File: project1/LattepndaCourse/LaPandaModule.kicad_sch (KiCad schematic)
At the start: 1 part

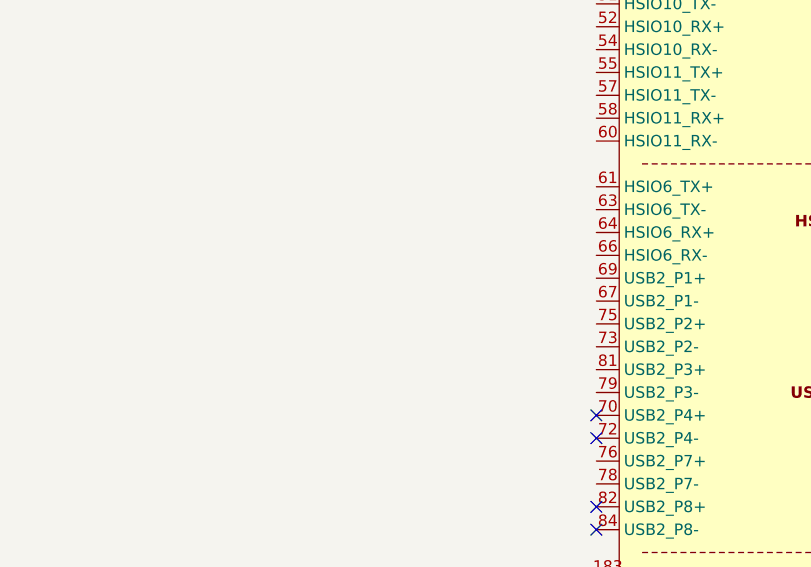
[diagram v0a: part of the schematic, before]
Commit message: test2
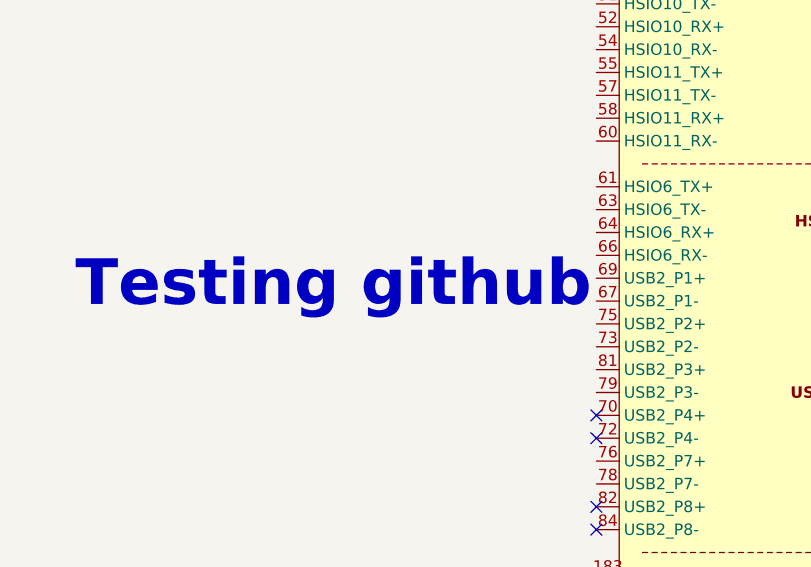
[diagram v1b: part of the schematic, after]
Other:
- note added: "Testing github"
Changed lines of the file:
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@@
 (kicad_sch
-	(version 20250114)
+	(version 20260306)
 	(generator "eeschema")
-	(generator_version "9.0")
+	(generator_version "10.0")
 	(paper "A2")
 	(title_block
@@
 		(rev "1")
 	)
+	(text "Testing github"
+		(exclude_from_sim no)
+		(at 226.06 181.102 0)
+		(effects
+			(font
+				(size 5.08 5.08)
+				(thickness 1.016)
+				(bold yes)
+				(color 255 51 215 1)
+			)
+		)
+	)
 	(no_connect
 		(at 255.27 195.58)
@@
 		(at 295.91 195.58 0)
 		(unit 1)
+		(body_style 1)
 		(exclude_from_sim no)
 		(in_bom yes)
 		(on_board yes)
+		(in_pos_files yes)
 		(dnp no)
 		(fields_autoplaced yes)
 		(property "Reference" "A1"
 			(at 300.5933 58.42 0)
+			(show_name no)
+			(do_not_autoplace no)
 			(effects
 				(font
@@
 		(property "Value" "LattePanda_Mu"
 			(at 300.5933 60.96 0)
+			(show_name no)
+			(do_not_autoplace no)
 			(effects
 				(font
@@
 		(property "Footprint" "Module_LattePanda:LattePanda_Module_H8.0mm_Horizontal"
 			(at 295.91 185.42 0)
+			(hide yes)
+			(show_name no)
+			(do_not_autoplace no)
 			(effects
 				(font
 					(size 1.27 1.27)
 				)
-				(hide yes)
 			)
 		)
 		(property "Datasheet" ""
 			(at 295.91 185.42 0)
+			(hide yes)
+			(show_name no)
+			(do_not_autoplace no)
 			(effects
 				(font
 					(size 1.27 1.27)
 				)
-				(hide yes)
 			)
 		)
 		(property "Description" "A micro computing module with x86 processer, RAM and eMMC."
 			(at 295.91 195.58 0)
+			(hide yes)
+			(show_name no)
+			(do_not_autoplace no)
 			(effects
 				(font
 					(size 1.27 1.27)
 				)
-				(hide yes)
 			)
 		)
@@
 		)
 		(instances
-			(project ""
+			(project "LattepndaCourse"
 				(path "/4e04f3a7-ba43-4db9-8bbc-1a27efcf5abf/e658b8ed-bbad-487b-848e-8e04e48b43c0"
 					(reference "A1")

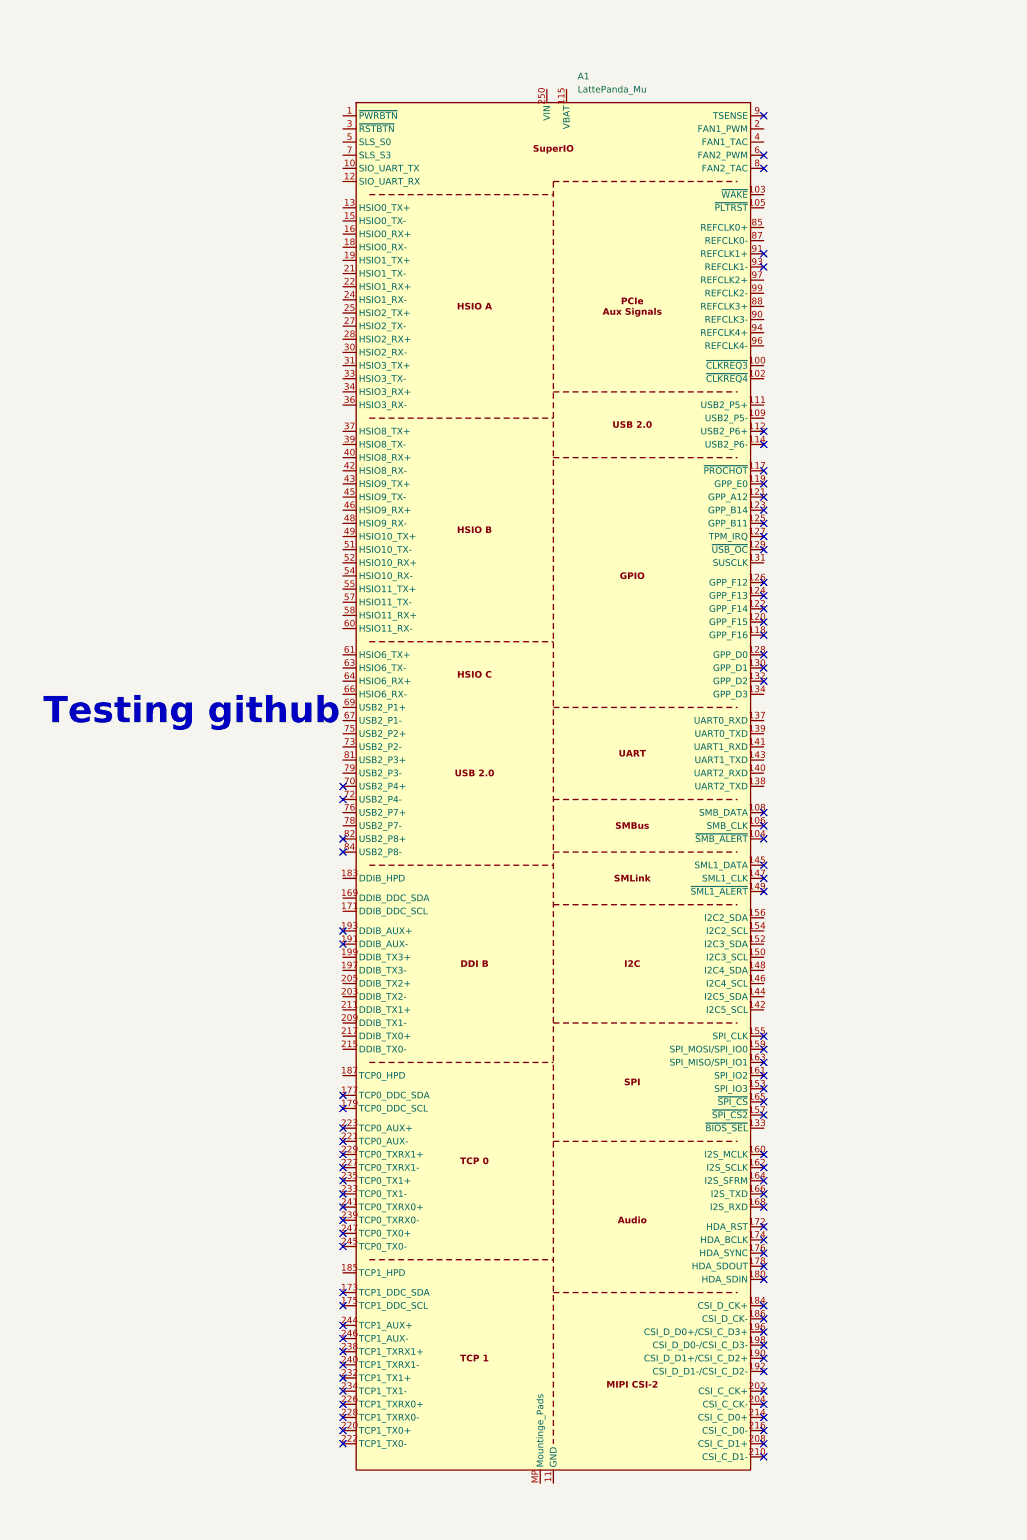
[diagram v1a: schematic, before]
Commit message: 9/30/36 10pm
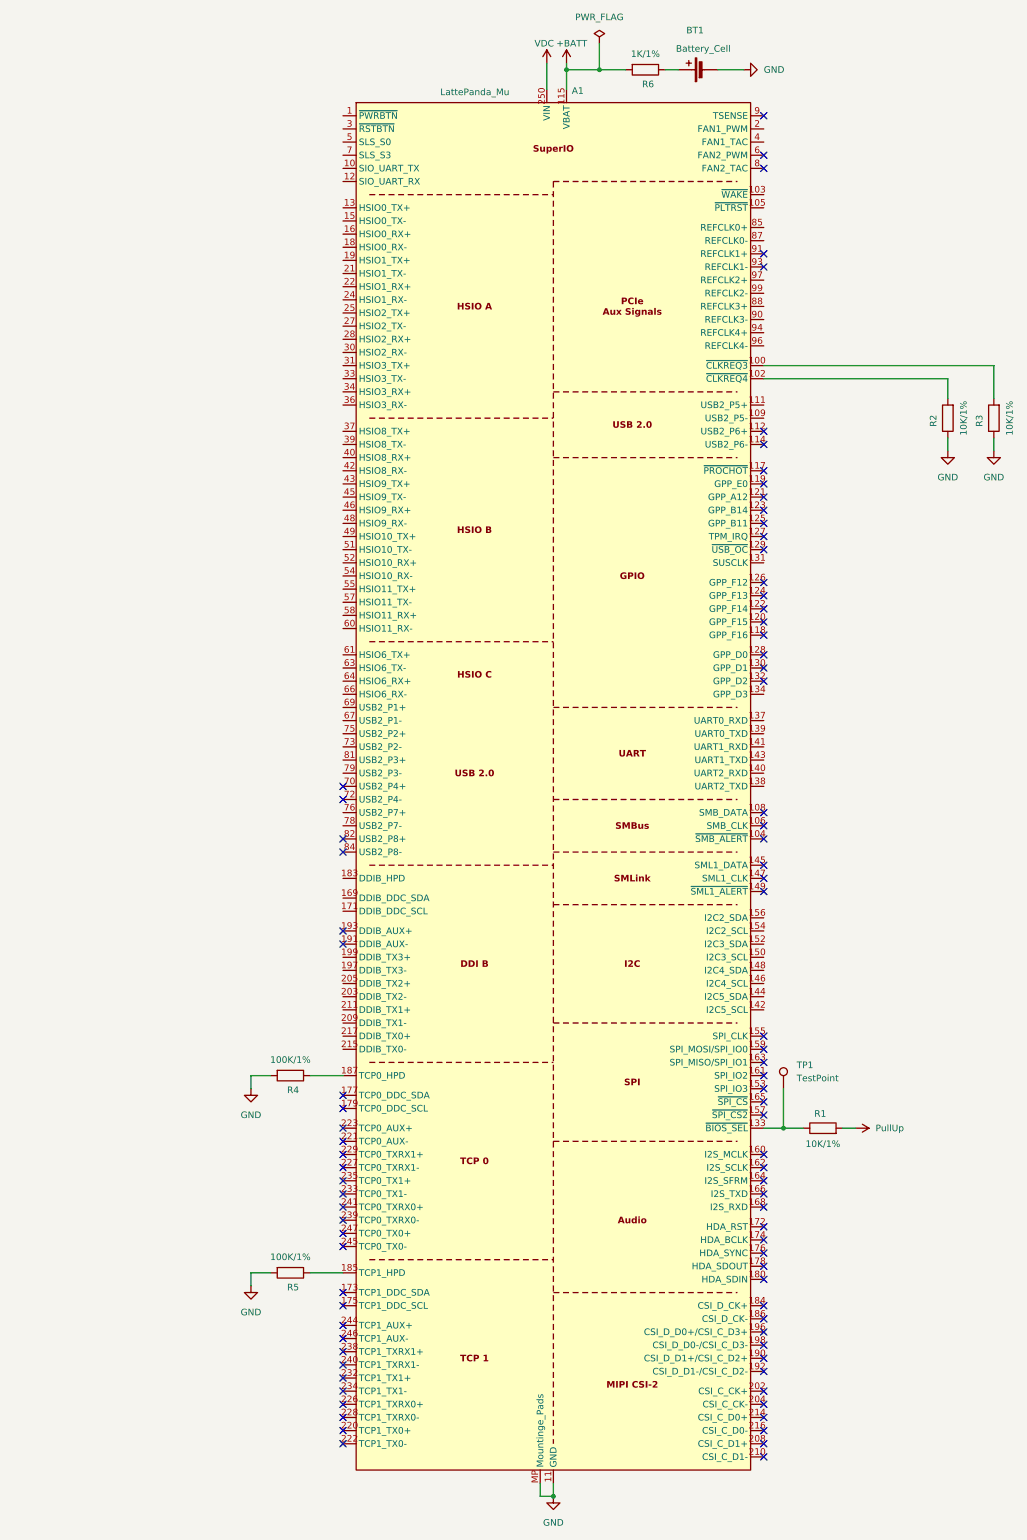
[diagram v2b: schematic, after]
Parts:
- added BT1: Battery_Cell, symbol Device:Battery_Cell
- added R1, R2, R3: 10K/1%, symbol Device:R
- added R4, R5: 100K/1%, symbol Device:R
- added R6: 1K/1%, symbol Device:R
- added TP1: TestPoint, symbol Connector:TestPoint
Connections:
- net at A1.100 (~{CLKREQ3}): now also R3.2
- net GND: now reaches A1.101 (GND), A1.107 (GND), A1.11 (GND), A1.110 (GND), A1.113 (GND), A1.116 (GND), A1.135 (GND), A1.136 (GND), A1.14 (GND), A1.151 (GND), A1.158 (GND), A1.167 (GND), A1.17 (GND), A1.170 (GND), A1.181 (GND), A1.182 (GND), A1.188 (GND), A1.189 (GND), A1.194 (GND), A1.195 (GND), A1.20 (GND), A1.200 (GND), A1.201 (GND), A1.206 (GND), A1.207 (GND), A1.212 (GND), A1.213 (GND), A1.218 (GND), A1.219 (GND), A1.224 (GND), A1.225 (GND), A1.23 (GND), A1.230 (GND), A1.231 (GND), A1.236 (GND), A1.237 (GND), A1.242 (GND), A1.243 (GND), A1.248 (GND), A1.249 (GND), A1.26 (GND), A1.29 (GND), A1.32 (GND), A1.35 (GND), A1.38 (GND), A1.41 (GND), A1.44 (GND), A1.47 (GND), A1.50 (GND), A1.53 (GND), A1.56 (GND), A1.59 (GND), A1.62 (GND), A1.65 (GND), A1.68 (GND), A1.71 (GND), A1.74 (GND), A1.77 (GND), A1.80 (GND), A1.83 (GND), A1.86 (GND), A1.89 (GND), A1.92 (GND), A1.95 (GND), A1.98 (GND)
- net GND: now also A1.MP (Mountinge_Pads), BT1.2 (-), R2.1, R3.1, R4.2, R5.2
- net at A1.102 (~{CLKREQ4}): now also R2.2
- net +BATT: now reaches A1.115 (VBAT)
- net +BATT: now also R6.2
- net at A1.133 (~{BIOS_SEL}): now also R1.1, TP1.1
- net at A1.185 (TCP1_HPD): now also R5.1
- net at A1.187 (TCP0_HPD): now also R4.1
- net VDC: now reaches A1.250 (VIN), A1.251 (VIN), A1.252 (VIN), A1.253 (VIN), A1.254 (VIN), A1.255 (VIN), A1.256 (VIN), A1.257 (VIN), A1.258 (VIN), A1.259 (VIN), A1.260 (VIN)
- new net: BT1.1 (+), R6.1
- new net PullUp: R1.2
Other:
- note removed: "Testing github"
